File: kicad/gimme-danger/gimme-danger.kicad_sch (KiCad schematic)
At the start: 62 parts, among them J2 Barrel_Jack, J3 Screw_Terminal_01x06, Q1 AO3400A, Q2 AO3400A, Q3 AO3400A, Q4 AO3400A, U1 ESP32-S3-WROOM-1, U10 AO4805, U11 DDTC143EUA, U2 TYPE-C-31-M-12, U3 TPD4E1U06DCKR, U5 SKRKAEE020, U7 SKRKAEE020, U8 TPS54302, U9 INA219AIDR

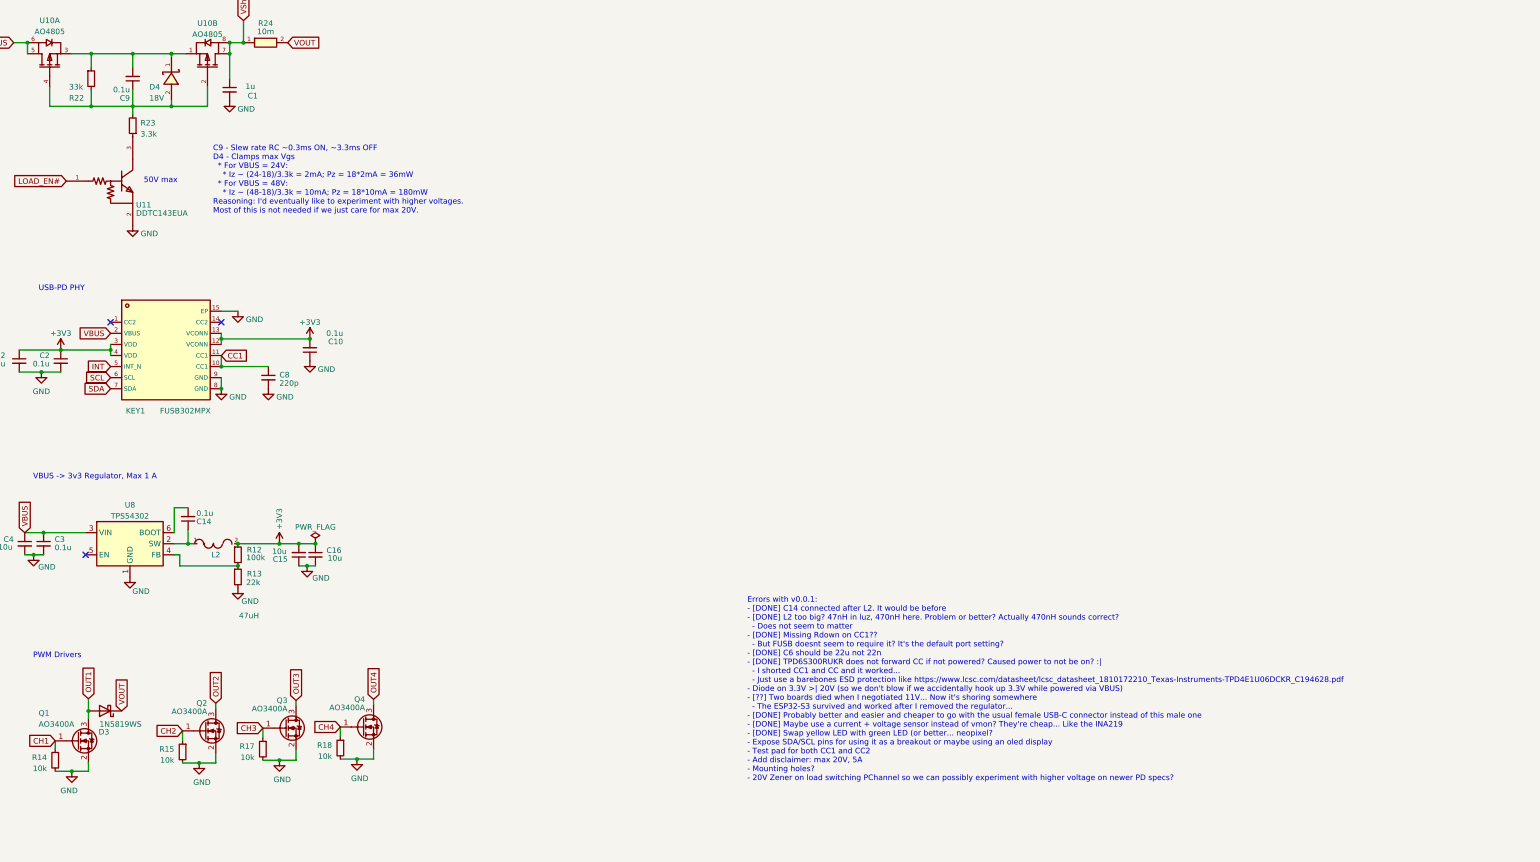
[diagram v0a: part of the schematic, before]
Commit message: Notes
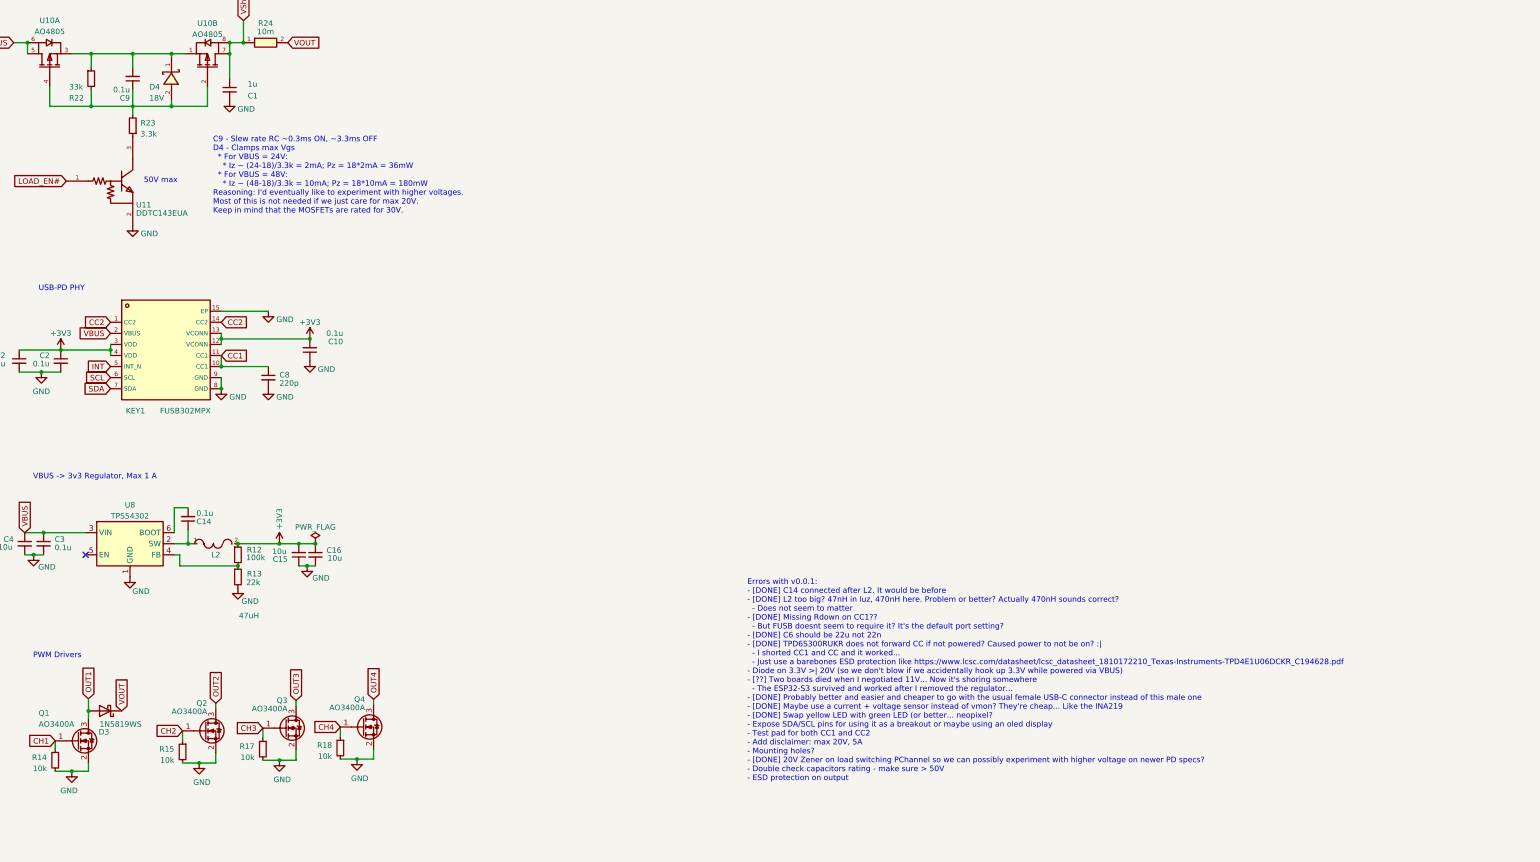
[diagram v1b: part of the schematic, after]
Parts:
- C1: footprint Capacitor_SMD:C_0402_1005Metric -> Capacitor_SMD:C_0603_1608Metric; LCSC C52923 -> C15849
- C4: footprint Capacitor_SMD:C_0603_1608Metric -> Capacitor_SMD:C_0805_2012Metric; LCSC C96446 -> C440198
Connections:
- net CC2: now also KEY1.1 (CC2), KEY1.14 (CC2)
- no-connect marks 33 -> 31
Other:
- note added: "C9 - Slew rate RC ~0.3ms ON, ~3.3ms OFF D4 - Clamps max Vgs * For VBUS = 24V: * Iz ~ (24-18)/3.3k = 2mA; Pz = 18*2mA = 36mW * For VBUS = 48V: * Iz ~ (48-18)/3.3k = 10mA; Pz = 18*10mA = 180mW Reasoning: I'd eventually like to experiment with higher voltages. Most of this is not needed if we just care for max 20V. Keep in mind that the MOSFETs are rated for 30V."
- note removed: "C9 - Slew rate RC ~0.3ms ON, ~3.3ms OFF D4 - Clamps max Vgs * For VBUS = 24V: * Iz ~ (24-18)/3.3k = 2mA; Pz = 18*2mA = 36mW * For VBUS = 48V: * Iz ~ (48-18)/3.3k = 10mA; Pz = 18*10mA = 180mW Reasoning: I'd eventually like to experiment with higher voltages. Most of this is not needed if we just care for max 20V."
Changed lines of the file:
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@@
   (no_connect (at 85.725 161.29))
   (no_connect (at 40.64 203.835))
-  (no_connect (at 313.055 95.885))
   (no_connect (at 43.18 203.835))
   (no_connect (at 281.94 149.225))
@@
   (no_connect (at 40.64 160.655))
   (no_connect (at 44.45 68.58))
-  (no_connect (at 287.655 95.885))
   (no_connect (at 135.89 116.84))
   (no_connect (at 135.89 81.28))
@@
     (stroke (width 0) (type default))
   )
-  (wire (pts (xy 313.055 93.345) (xy 316.865 93.345))
+  (wire (pts (xy 313.055 93.345) (xy 323.85 93.345))
     (stroke (width 0) (type default))
   )
@@
     (effects (font (size 1.27 1.27)) (justify left bottom))
   )
-  (text "Errors with v0.0.1:\n- [DONE] C14 connected after L2. It would be before\n- [DONE] L2 too big? 47nH in luz, 470nH here. Problem or better? Actually 470nH sounds correct?\n  - Does not seem to matter\n- [DONE] Missing Rdown on CC1??\n  - But FUSB doesnt seem to require it? It's the default port setting?\n- [DONE] C6 should be 22u not 22n\n- [DONE] TPD6S300RUKR does not forward CC if not powered? Caused power to not be on? :|\n  - I shorted CC1 and CC and it worked...\n  - Just use a barebones ESD protection like https://www.lcsc.com/datasheet/lcsc_datasheet_1810172210_Texas-Instruments-TPD4E1U06DCKR_C194628.pdf\n- Diode on 3.3V >| 20V (so we don't blow if we accidentally hook up 3.3V while powered via VBUS)\n- [??] Two boards died when I negotiated 11V... Now it's shoring somewhere\n  - The ESP32-S3 survived and worked after I removed the regulator...\n- [DONE] Probably better and easier and cheaper to go with the usual female USB-C connector instead of this male one\n- [DONE] Maybe use a current + voltage sensor instead of vmon? They're cheap... Like the INA219\n- [DONE] Swap yellow LED with green LED (or better... neopixel?\n- Expose SDA/SCL pins for using it as a breakout or maybe using an oled display\n- Test pad for both CC1 and CC2\n- Add disclaimer: max 20V, 5A\n- Mounting holes?\n- 20V Zener on load switching PChannel so we can possibly experiment with higher voltage on newer PD specs?"
+  (text "Errors with v0.0.1:\n- [DONE] C14 connected after L2. It would be before\n- [DONE] L2 too big? 47nH in luz, 470nH here. Problem or better? Actually 470nH sounds correct?\n  - Does not seem to matter\n- [DONE] Missing Rdown on CC1??\n  - But FUSB doesnt seem to require it? It's the default port setting?\n- [DONE] C6 should be 22u not 22n\n- [DONE] TPD6S300RUKR does not forward CC if not powered? Caused power to not be on? :|\n  - I shorted CC1 and CC and it worked...\n  - Just use a barebones ESD protection like https://www.lcsc.com/datasheet/lcsc_datasheet_1810172210_Texas-Instruments-TPD4E1U06DCKR_C194628.pdf\n- Diode on 3.3V >| 20V (so we don't blow if we accidentally hook up 3.3V while powered via VBUS)\n- [??] Two boards died when I negotiated 11V... Now it's shoring somewhere\n  - The ESP32-S3 survived and worked after I removed the regulator...\n- [DONE] Probably better and easier and cheaper to go with the usual female USB-C connector instead of this male one\n- [DONE] Maybe use a current + voltage sensor instead of vmon? They're cheap... Like the INA219\n- [DONE] Swap yellow LED with green LED (or better... neopixel?\n- Expose SDA/SCL pins for using it as a breakout or maybe using an oled display\n- Test pad for both CC1 and CC2\n- Add disclaimer: max 20V, 5A\n- Mounting holes?\n- [DONE] 20V Zener on load switching PChannel so we can possibly experiment with higher voltage on newer PD specs?\n- Double check capacitors rating - make sure > 50V\n- ESD protection on output"
     (at 433.705 201.295 0)
     (effects (font (size 1.27 1.27)) (justify left bottom))
@@
     (effects (font (size 1.27 1.27)) (justify left bottom))
   )
-  (text "C9 - Slew rate RC ~0.3ms ON, ~3.3ms OFF\nD4 - Clamps max Vgs\n  * For VBUS = 24V:\n    * Iz ~ (24-18)/3.3k = 2mA; Pz = 18*2mA = 36mW\n  * For VBUS = 48V:\n    * Iz ~ (48-18)/3.3k = 10mA; Pz = 18*10mA = 180mW\nReasoning: I'd eventually like to experiment with higher voltages.\nMost of this is not needed if we just care for max 20V."
+  (text "C9 - Slew rate RC ~0.3ms ON, ~3.3ms OFF\nD4 - Clamps max Vgs\n  * For VBUS = 24V:\n    * Iz ~ (24-18)/3.3k = 2mA; Pz = 18*2mA = 36mW\n  * For VBUS = 48V:\n    * Iz ~ (48-18)/3.3k = 10mA; Pz = 18*10mA = 180mW\nReasoning: I'd eventually like to experiment with higher voltages.\nMost of this is not needed if we just care for max 20V.\nKeep in mind that the MOSFETs are rated for 30V."
     (at 311.15 71.12 0)
     (effects (font (size 1.27 1.27)) (justify left bottom))
@@
     )
   )
+  (global_label "CC2" (shape input) (at 313.055 95.885 0) (fields_autoplaced)
+    (effects (font (size 1.27 1.27)) (justify left))
+    (property "Intersheetrefs" "${INTERSHEET_REFS}" (at 319.7103 95.885 0)
+      (effects (font (size 1.27 1.27)) (justify left) hide)
+    )
+  )
   (global_label "VOUT" (shape input) (at 328.295 31.75 0) (fields_autoplaced)
     (effects (font (size 1.27 1.27)) (justify left))
@@
     (effects (font (size 1.27 1.27)) (justify right))
     (property "Intersheetrefs" "${INTERSHEET_REFS}" (at 281.8463 106.045 0)
+      (effects (font (size 1.27 1.27)) (justify right) hide)
+    )
+  )
+  (global_label "CC2" (shape input) (at 287.655 95.885 180) (fields_autoplaced)
+    (effects (font (size 1.27 1.27)) (justify right))
+    (property "Intersheetrefs" "${INTERSHEET_REFS}" (at 280.9997 95.885 0)
       (effects (font (size 1.27 1.27)) (justify right) hide)
     )
@@
       (effects (font (size 1.27 1.27)) (justify left))
     )
-    (property "Footprint" "Capacitor_SMD:C_0603_1608Metric" (at 267.97 146.685 0)
+    (property "Footprint" "Capacitor_SMD:C_0805_2012Metric" (at 267.97 146.685 0)
       (effects (font (size 1.27 1.27)) hide)
     )
@@
       (effects (font (size 1.27 1.27)) hide)
     )
-    (property "LCSC" "C96446" (at 267.97 146.685 0)
+    (property "LCSC" "C440198" (at 267.97 146.685 0)
       (effects (font (size 1.27 1.27)) hide)
     )
@@
       (effects (font (size 1.27 1.27)) (justify left))
     )
-    (property "Value" "1u" (at 320.802 41.783 0)
-      (effects (font (size 1.27 1.27)) (justify left))
-    )
-    (property "Footprint" "Capacitor_SMD:C_0402_1005Metric" (at 314.96 42.545 0)
+    (property "Value" "1u" (at 321.31 41.275 0)
+      (effects (font (size 1.27 1.27)) (justify left))
+    )
+    (property "Footprint" "Capacitor_SMD:C_0603_1608Metric" (at 314.96 42.545 0)
       (effects (font (size 1.27 1.27)) hide)
     )
@@
       (effects (font (size 1.27 1.27)) hide)
     )
-    (property "LCSC" "C52923" (at 314.96 42.545 0)
+    (property "LCSC" "C15849" (at 314.96 42.545 0)
       (effects (font (size 1.27 1.27)) hide)
     )
@@
     )
   )
-  (symbol (lib_id "power:GND") (at 316.865 93.345 0) (unit 1)
-    (in_bom yes) (on_board yes) (dnp no)
-    (property "Reference" "#PWR015" (at 316.865 99.695 0)
-      (effects (font (size 1.27 1.27)) hide)
-    )
-    (property "Value" "GND" (at 320.675 95.25 0)
-      (effects (font (size 1.27 1.27)))
-    )
-    (property "Footprint" "" (at 316.865 93.345 0)
-      (effects (font (size 1.27 1.27)) hide)
-    )
-    (property "Datasheet" "" (at 316.865 93.345 0)
-      (effects (font (size 1.27 1.27)) hide)
-    )
+  (symbol (lib_id "power:GND") (at 323.85 93.345 0) (unit 1)
+    (in_bom yes) (on_board yes) (dnp no)
+    (property "Reference" "#PWR015" (at 323.85 99.695 0)
+      (effects (font (size 1.27 1.27)) hide)
+    )
+    (property "Value" "GND" (at 327.66 95.25 0)
+      (effects (font (size 1.27 1.27)))
+    )
+    (property "Footprint" "" (at 323.85 93.345 0)
+      (effects (font (size 1.27 1.27)) hide)
+    )
+    (property "Datasheet" "" (at 323.85 93.345 0)
+      (effects (font (size 1.27 1.27)) hide)
+    )

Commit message: TVS diodes on output
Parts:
- removed D3: 1N5819WS, Diode_SMD:D_SOD-323, symbol Diode:1N5819WS
- removed J2: Barrel_Jack, symbol Connector:Barrel_Jack
- removed U10: AO4805, footprint:SOIC-8_L4.9-W3.9-P1.27-LS6.0-BL, symbol AO4805:AO4805
- added D3, D5, D7, D8: SMAJ28A, footprint:SMA_L4.3-W2.6-LS5.2-RD, symbol SMAJ28A_C283899:SMAJ28A_C283899
- added D6: SMAJ48A, footprint:SMA_L4.3-W2.5-LS5.0-RD, symbol SMAJ48A_C353444:SMAJ48A_C353444
- added REF1, REF2: DMP6023LE-13, footprint:SOT-223-4_L6.5-W3.5-P2.30-LS7.0-BR, symbol DMP6023LE-13:DMP6023LE-13
- added U4: DC-84, footprint:DC-IN-TH_DC-84, symbol DC-84:DC-84
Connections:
- net GND: now also D6.2 (A), U4.2, U4.3
- net OUT1: now also D5.2
- net OUT2: now also D8.2
- net OUT3: now also D3.2
- net OUT4: now also D7.2
- net VBUS: now also REF1.2 (D), REF1.4 (D)
- net VOUT: now also D3.1, D5.1, D6.1 (C), D7.1, D8.1, U4.1
- net VSh+: now also REF2.2 (D), REF2.4 (D)
- net at C9.2, D4.1 (K), R22.1: now also REF1.3 (S), REF2.3 (S)
- net at C9.1, D4.2 (A), R22.2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: now also REF1.1 (G), REF2.1 (G)
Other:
- note added: "TODO - USB resistors (for termination + protection? 100 Ohm?) - [DONE] Voltage monitor? - [DONE] CC test pad - [DONE] Decoupling caps on CC line? How big? FUSB302 datasheet says 200 - 600 pF - [DONE] Make sure caps on VBUS/VINT support > 20V (what about surges?) - [DONE] TVS on VOUT -- eg. if we want to drive an inductive load with safety flyback? Maybe SMF22"
- note removed: "TODO - USB resistors (for termination + protection? 100 Ohm?) - [DONE] Voltage monitor? - [DONE] CC test pad - [DONE] Decoupling caps on CC line? How big? FUSB302 datasheet says 200 - 600 pF - Make sure caps on VBUS/VINT support > 20V (what about surges?) - TVS on VOUT -- eg. if we want to drive an inductive load with safety flyback? Maybe SMF22"
- moved on the sheet: C1, Q3, Q4, R17, R18, R24
